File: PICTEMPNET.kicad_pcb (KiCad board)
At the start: 2 copper layers, 123.9 x 52.7 mm, 75 parts, among them J1 Barrel Jack, J2 08B0-1X1T-36-F, J3 RJ-12, J4 LCM-S01602DTR_M, SW1 SW_Push, U1 PIC18F97J60-IPT, U2 LM2940S-5.0/NOPB, U3 TC1262-3.3, U4 ENC28J60x-ML, U5 TC1047xNB, Y1 25 MHz, Y2 32 kHz, Y3 25 MHz

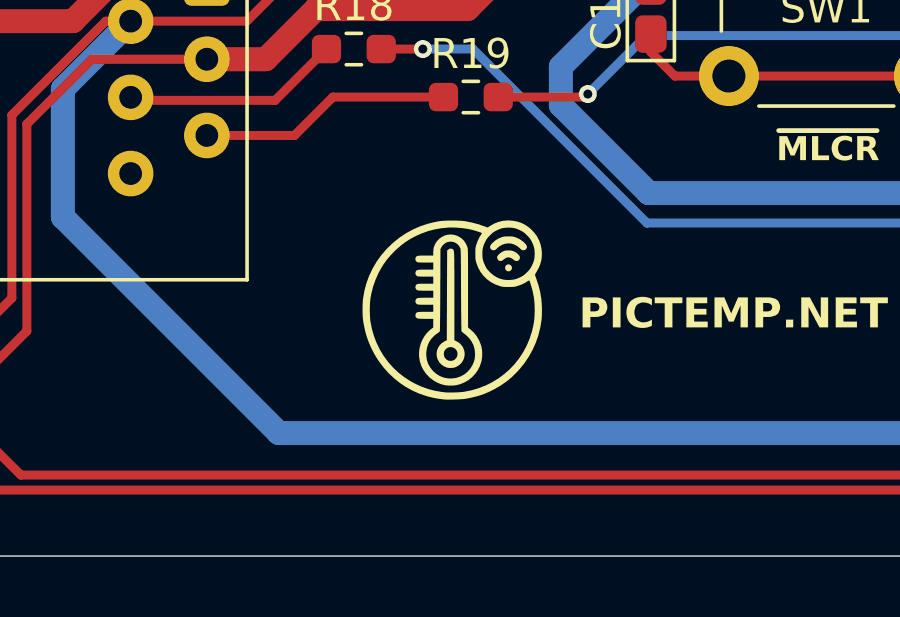
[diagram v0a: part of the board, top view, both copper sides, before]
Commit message: KiCAD files
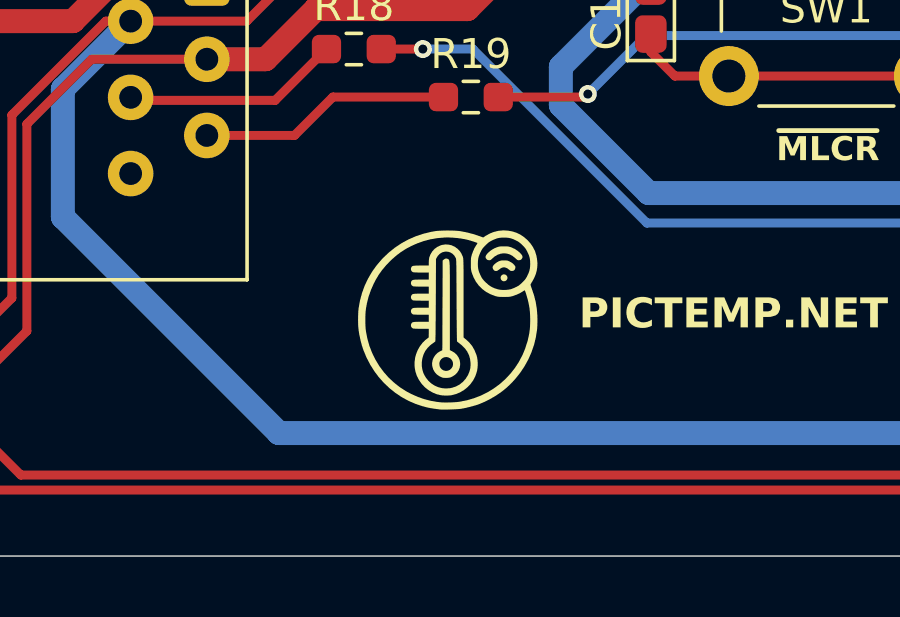
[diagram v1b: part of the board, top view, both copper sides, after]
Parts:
- moved LOGO 0.63 mm to (108.5, 124.0)
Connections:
- net +9V renamed /+9V
- J4 pad 15: NC0 -> unconnected-(J4-LED+-Pad15)
- J4 pad 16: NC1 -> unconnected-(J4-LED--Pad16)
